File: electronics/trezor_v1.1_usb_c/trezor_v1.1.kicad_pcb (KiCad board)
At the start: 2 copper layers, 50 x 26.7 mm, 34 parts, among them IC1 MCP1703T-3302E/CB, J1 USB_C_Receptacle_USB2.0, K2 SWD, Q2 8MHz, U1 STM32F205RET6, U3 DISPLAY

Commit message: kicad: update project to kicad 6
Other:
- net class Default removed

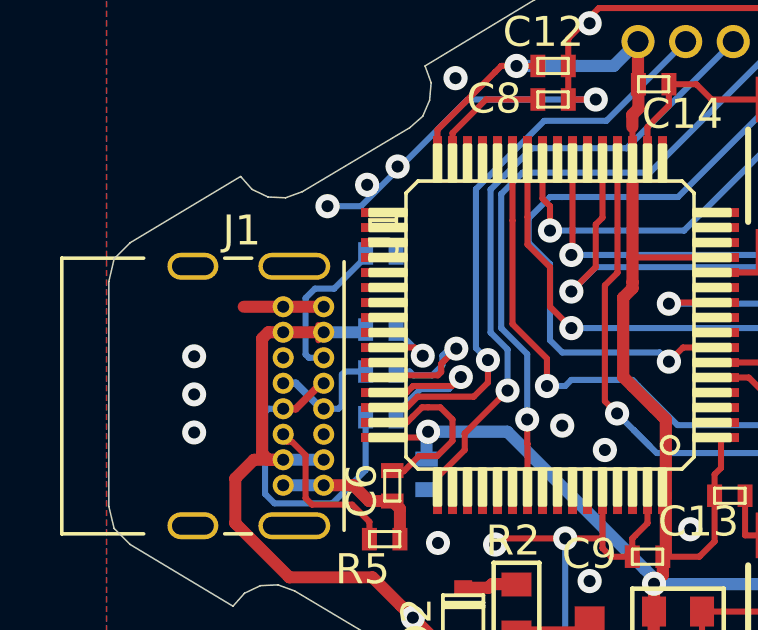
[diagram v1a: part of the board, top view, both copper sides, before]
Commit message: cleanup: fix 3d models in pcb
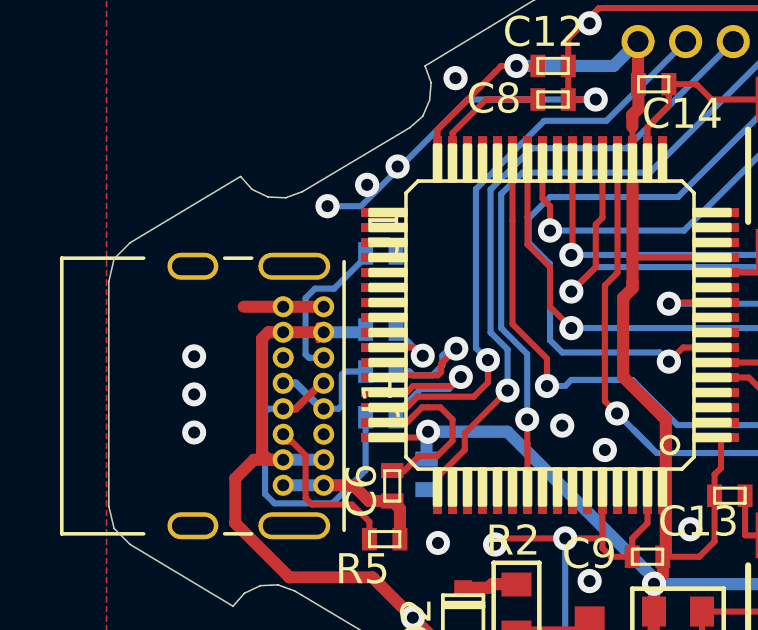
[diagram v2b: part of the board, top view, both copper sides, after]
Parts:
- J1: footprint Connector_USB:USB_C_Receptacle_GCT_USB4085 -> Gigahawk:USB_C_Receptacle_GCT_USB4085
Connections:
- J1 pad A8: Net-(J1-PadA8) -> unconnected-(J1-PadA8)
- J1 pad B8: Net-(J1-PadB8) -> unconnected-(J1-PadB8)
- U1 pad 11: Net-(U1-Pad11) -> unconnected-(U1-Pad11)
- U1 pad 14: Net-(U1-Pad14) -> unconnected-(U1-Pad14)
- U1 pad 15: Net-(U1-Pad15) -> unconnected-(U1-Pad15)
- U1 pad 16: Net-(U1-Pad16) -> unconnected-(U1-Pad16)
- U1 pad 17: Net-(U1-Pad17) -> unconnected-(U1-Pad17)
- U1 pad 22: Net-(U1-Pad22) -> unconnected-(U1-Pad22)
- U1 pad 24: Net-(U1-Pad24) -> unconnected-(U1-Pad24)
- U1 pad 28: Net-(U1-Pad28) -> unconnected-(U1-Pad28)
- U1 pad 37: Net-(U1-Pad37) -> unconnected-(U1-Pad37)
- U1 pad 38: Net-(U1-Pad38) -> unconnected-(U1-Pad38)
- U1 pad 41: Net-(U1-Pad41) -> unconnected-(U1-Pad41)
- U1 pad 43: Net-(U1-Pad43) -> unconnected-(U1-Pad43)
- U1 pad 50: Net-(U1-Pad50) -> unconnected-(U1-Pad50)
- U1 pad 54: Net-(U1-Pad54) -> unconnected-(U1-Pad54)
- U1 pad 56: Net-(U1-Pad56) -> unconnected-(U1-Pad56)
- U1 pad 57: Net-(U1-Pad57) -> unconnected-(U1-Pad57)
- U1 pad 58: Net-(U1-Pad58) -> unconnected-(U1-Pad58)
- U1 pad 59: Net-(U1-Pad59) -> unconnected-(U1-Pad59)
- U1 pad 8: Net-(U1-Pad8) -> unconnected-(U1-Pad8)
- U1 pad 9: Net-(U1-Pad9) -> unconnected-(U1-Pad9)
- U3 pad 16: Net-(U3-Pad16) -> unconnected-(U3-Pad16)
- U3 pad 17: Net-(U3-Pad17) -> unconnected-(U3-Pad17)
- U3 pad 20: Net-(U3-Pad20) -> unconnected-(U3-Pad20)
- U3 pad 21: Net-(U3-Pad21) -> unconnected-(U3-Pad21)
- U3 pad 22: Net-(U3-Pad22) -> unconnected-(U3-Pad22)
- U3 pad 23: Net-(U3-Pad23) -> unconnected-(U3-Pad23)
- U3 pad 24: Net-(U3-Pad24) -> unconnected-(U3-Pad24)
- U3 pad 25: Net-(U3-Pad25) -> unconnected-(U3-Pad25)
- U3 pad 7: Net-(U3-Pad7) -> unconnected-(U3-Pad7)
